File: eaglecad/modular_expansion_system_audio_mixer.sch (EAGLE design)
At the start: 82 parts, among them IC1 TL084P, J1 RCA, J1_ADDRESS_CON j1, J2 RCA, J2_DATA_AND_POWER_CON j2, J3 RCA, J4 RCA, J5 RCA, X1 STEREOJACK

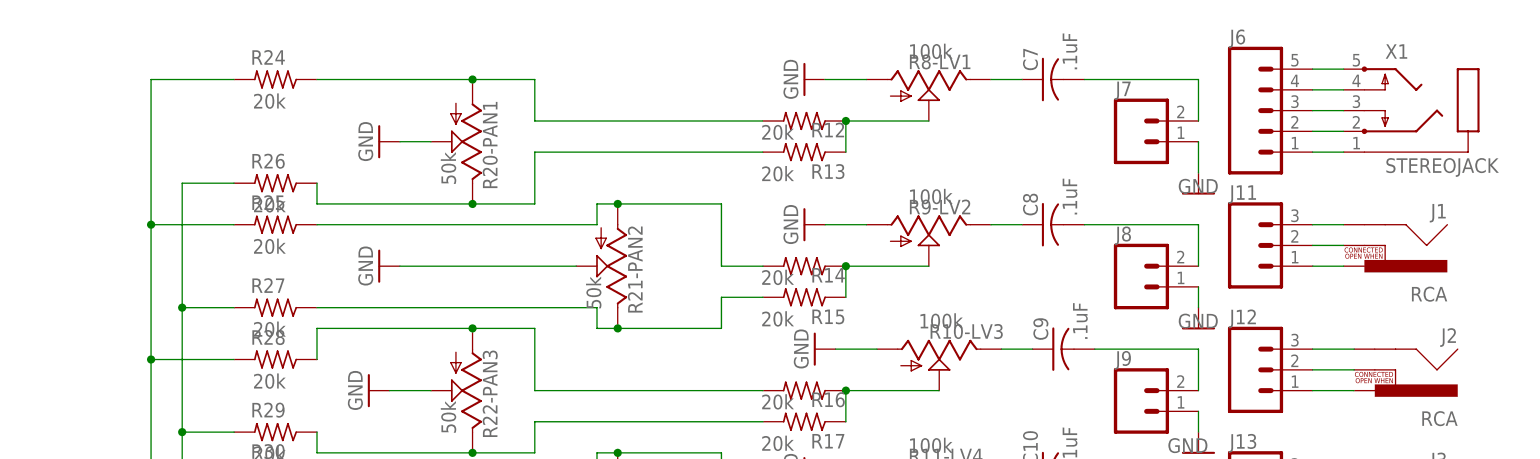
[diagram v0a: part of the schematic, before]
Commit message: various fixes
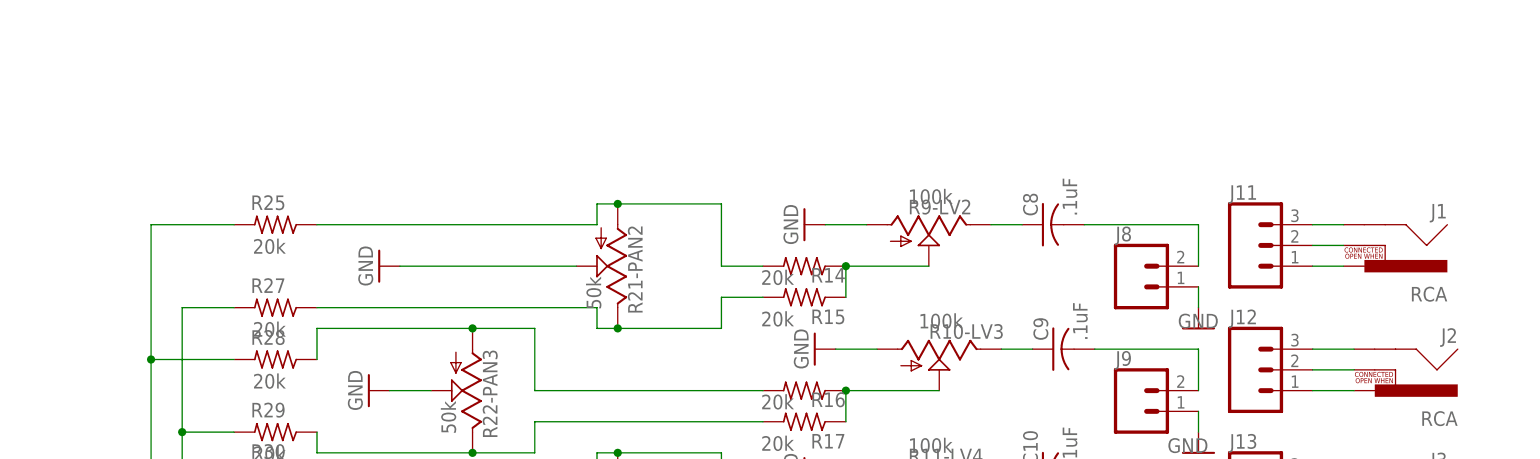
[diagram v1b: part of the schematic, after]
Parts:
- removed C7: .1uF, rcl:C-US025-024X044
- removed J6: (no value), SparkFun-Connectors:CONN_05
- removed J7: (no value), SparkFun-Connectors:CONN_02
- removed R12, R13, R24, R26: 20k, resistor:R-US_0204/2V
- removed R20-PAN1: 50k, pot:TRIM_US-B25U
- removed R8-LV1: 100k, pot:TRIM_US-B25U
- removed X1: STEREOJACK, audio amplifier example:STEREOJACK
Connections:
- removed net N$10: J6.5, X1.5
- removed net N$11: J6.4, X1.4
- removed net N$12: J6.3, X1.3
- removed net N$13: J6.2, X1.2
- removed net N$14: J6.1, X1.1
- removed net N$30: C7.1, R8-LV1.E
- removed net N$34: C7.2, J7.2
- removed net N$38: R12.1, R13.1, R8-LV1.S
- removed net N$42: R13.2, R20-PAN1.E, R26.1
- removed net N$43: R12.2, R20-PAN1.A, R24.1
- net GND: no longer J7.1, R20-PAN1.S, R8-LV1.A
- net N$51: no longer R24.2
- net N$54: no longer R26.2
